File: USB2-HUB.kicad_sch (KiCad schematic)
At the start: 30 parts, among them IC2 TPS2553QDBVRQ1, IC7 TPS2553QDBVRQ1, J4 USB_C_Receptacle_USB2.0_16P, J5 USB_C_Receptacle_USB2.0_16P, U3 FSUSB42MUX

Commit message: layout draft
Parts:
- J4, J5: footprint (none) -> Connector_USB:USB_C_Receptacle_GCT_USB4105-xx-A_16P_TopMnt_Horizontal
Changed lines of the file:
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@@
 			)
 		)
-		(property "Footprint" ""
+		(property "Footprint" "Connector_USB:USB_C_Receptacle_GCT_USB4105-xx-A_16P_TopMnt_Horizontal"
 			(at 256.54 41.91 0)
 			(effects
@@
 			)
 		)
-		(property "Footprint" ""
+		(property "Footprint" "Connector_USB:USB_C_Receptacle_GCT_USB4105-xx-A_16P_TopMnt_Horizontal"
 			(at 256.54 116.84 0)
 			(effects

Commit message: moved everything to front & 0603'd stuff
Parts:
- C1, C12, C13, C15, C16, C17, C2, C4, C50, C57: footprint Capacitor_SMD:C_0805_2012Metric -> Capacitor_SMD:C_0603_1608Metric
- R10, R11, R12, R3, R37, R38, R5, R6, R62, R69, R9: footprint Resistor_SMD:R_0805_2012Metric -> Resistor_SMD:R_0603_1608Metric
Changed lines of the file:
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@@
 			)
 		)
-		(property "Footprint" "Capacitor_SMD:C_0805_2012Metric"
+		(property "Footprint" "Capacitor_SMD:C_0603_1608Metric"
 			(at 251.1552 149.86 0)
 			(effects
@@
 			)
 		)
-		(property "Footprint" "Resistor_SMD:R_0805_2012Metric"
+		(property "Footprint" "Resistor_SMD:R_0603_1608Metric"
 			(at 156.21 57.658 90)
 			(effects
@@
 			)
 		)
-		(property "Footprint" "Resistor_SMD:R_0805_2012Metric"
+		(property "Footprint" "Resistor_SMD:R_0603_1608Metric"
 			(at 204.978 57.15 90)
 			(effects
@@
 			)
 		)
-		(property "Footprint" "Resistor_SMD:R_0805_2012Metric"
+		(property "Footprint" "Resistor_SMD:R_0603_1608Metric"
 			(at 156.21 132.588 90)
 			(effects
@@
 			)
 		)
-		(property "Footprint" "Resistor_SMD:R_0805_2012Metric"
+		(property "Footprint" "Resistor_SMD:R_0603_1608Metric"
 			(at 241.3 29.972 90)
 			(effects
@@
 			)
 		)
-		(property "Footprint" "Capacitor_SMD:C_0805_2012Metric"
+		(property "Footprint" "Capacitor_SMD:C_0603_1608Metric"
 			(at 163.5252 64.77 0)
 			(effects
@@
 			)
 		)
-		(property "Footprint" "Capacitor_SMD:C_0805_2012Metric"
+		(property "Footprint" "Capacitor_SMD:C_0603_1608Metric"
 			(at 163.5252 139.7 0)
 			(effects
@@
 			)
 		)
-		(property "Footprint" "Resistor_SMD:R_0805_2012Metric"
+		(property "Footprint" "Resistor_SMD:R_0603_1608Metric"
 			(at 241.3 32.512 90)
 			(effects
@@
 			)
 		)
-		(property "Footprint" "Resistor_SMD:R_0805_2012Metric"
+		(property "Footprint" "Resistor_SMD:R_0603_1608Metric"
 			(at 241.3 104.902 90)
 			(effects
@@
 			)
 		)
-		(property "Footprint" "Resistor_SMD:R_0805_2012Metric"
+		(property "Footprint" "Resistor_SMD:R_0603_1608Metric"
 			(at 232.918 146.05 90)
 			(effects
@@
 			)
 		)
-		(property "Footprint" "Capacitor_SMD:C_0805_2012Metric"
+		(property "Footprint" "Capacitor_SMD:C_0603_1608Metric"
 			(at 240.9952 74.93 0)
 			(effects
@@
 			)
 		)
-		(property "Footprint" "Capacitor_SMD:C_0805_2012Metric"
+		(property "Footprint" "Capacitor_SMD:C_0603_1608Metric"
 			(at 166.0652 119.38 0)
 			(effects
@@
 			)
 		)
-		(property "Footprint" "Capacitor_SMD:C_0805_2012Metric"
+		(property "Footprint" "Capacitor_SMD:C_0603_1608Metric"
 			(at 214.3252 34.29 0)
 			(effects
@@
 			)
 		)
-		(property "Footprint" "Capacitor_SMD:C_0805_2012Metric"
+		(property "Footprint" "Capacitor_SMD:C_0603_1608Metric"
 			(at 251.1552 74.93 0)
 			(effects
@@
 			)
 		)
-		(property "Footprint" "Capacitor_SMD:C_0805_2012Metric"
+		(property "Footprint" "Capacitor_SMD:C_0603_1608Metric"
 			(at 166.0652 44.45 0)
 			(effects
@@
 			)
 		)
-		(property "Footprint" "Resistor_SMD:R_0805_2012Metric"
+		(property "Footprint" "Resistor_SMD:R_0603_1608Metric"
 			(at 241.3 107.442 90)
 			(effects
@@
 			)
 		)
-		(property "Footprint" "Capacitor_SMD:C_0805_2012Metric"
+		(property "Footprint" "Capacitor_SMD:C_0603_1608Metric"
 			(at 240.9952 149.86 0)
 			(effects
@@
 			)
 		)
-		(property "Footprint" "Resistor_SMD:R_0805_2012Metric"
+		(property "Footprint" "Resistor_SMD:R_0603_1608Metric"
 			(at 36.322 171.45 90)
 			(effects
@@
 			)
 		)
-		(property "Footprint" "Resistor_SMD:R_0805_2012Metric"
+		(property "Footprint" "Resistor_SMD:R_0603_1608Metric"
 			(at 204.978 132.08 90)
 			(effects
@@
 			)
 		)
-		(property "Footprint" "Resistor_SMD:R_0805_2012Metric"
+		(property "Footprint" "Resistor_SMD:R_0603_1608Metric"
 			(at 232.918 71.12 90)
 			(effects
@@
 			)
 		)
-		(property "Footprint" "Capacitor_SMD:C_0805_2012Metric"
+		(property "Footprint" "Capacitor_SMD:C_0603_1608Metric"
 			(at 214.3252 109.22 0)
 			(effects

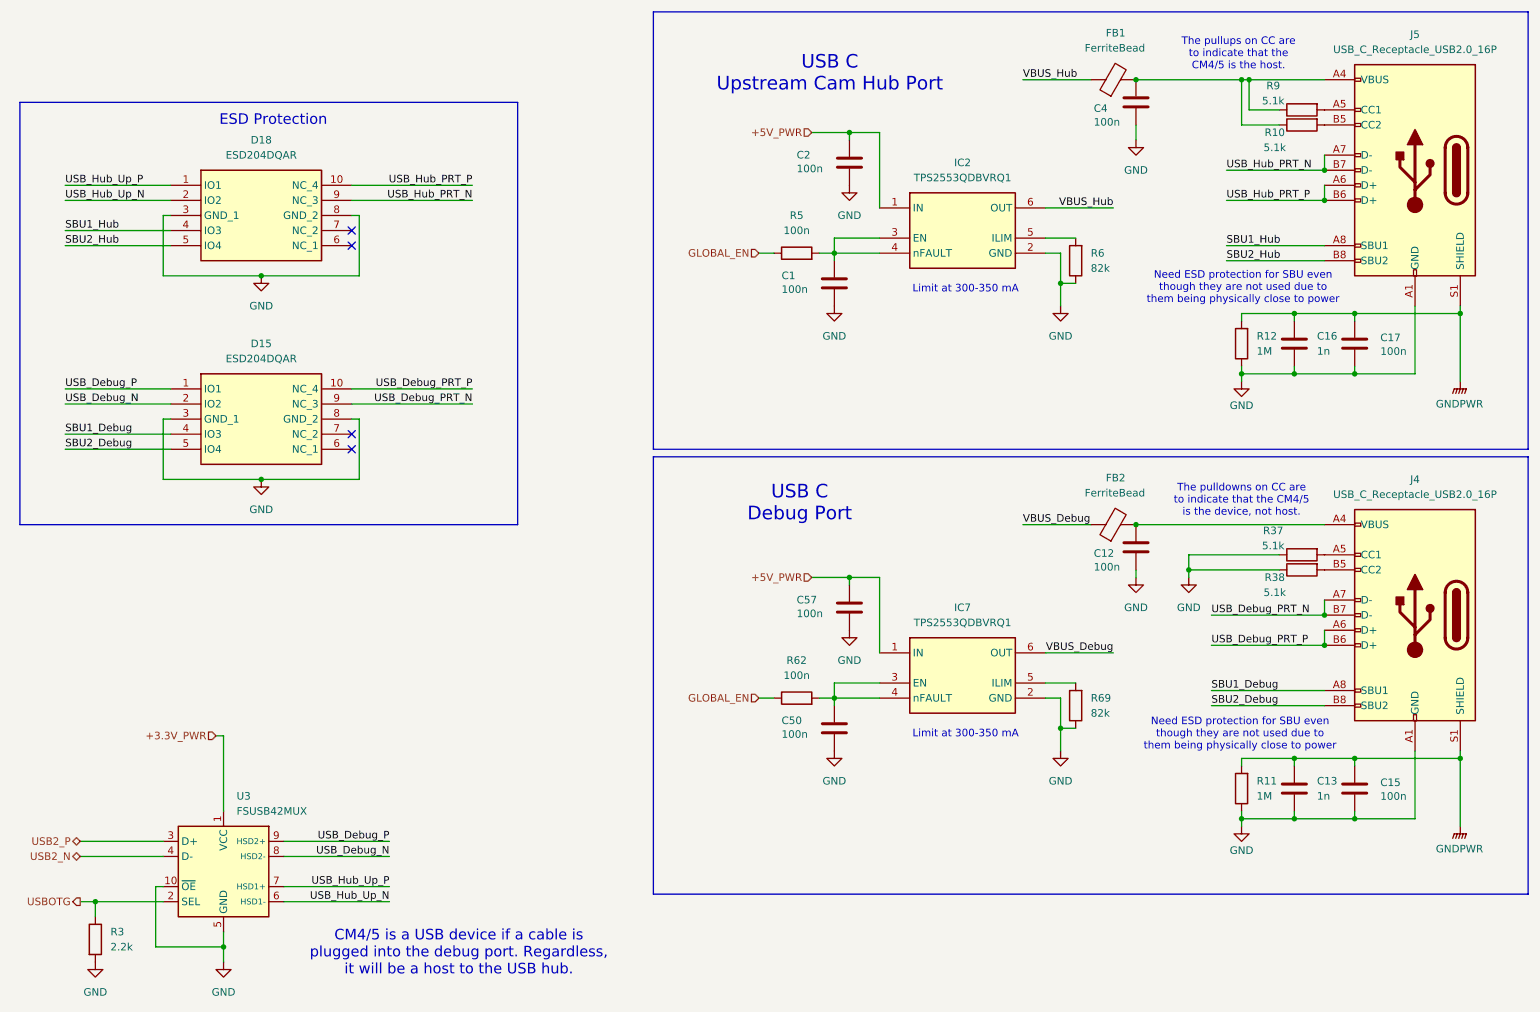
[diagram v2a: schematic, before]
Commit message: changed a bunch of stuff, still have work
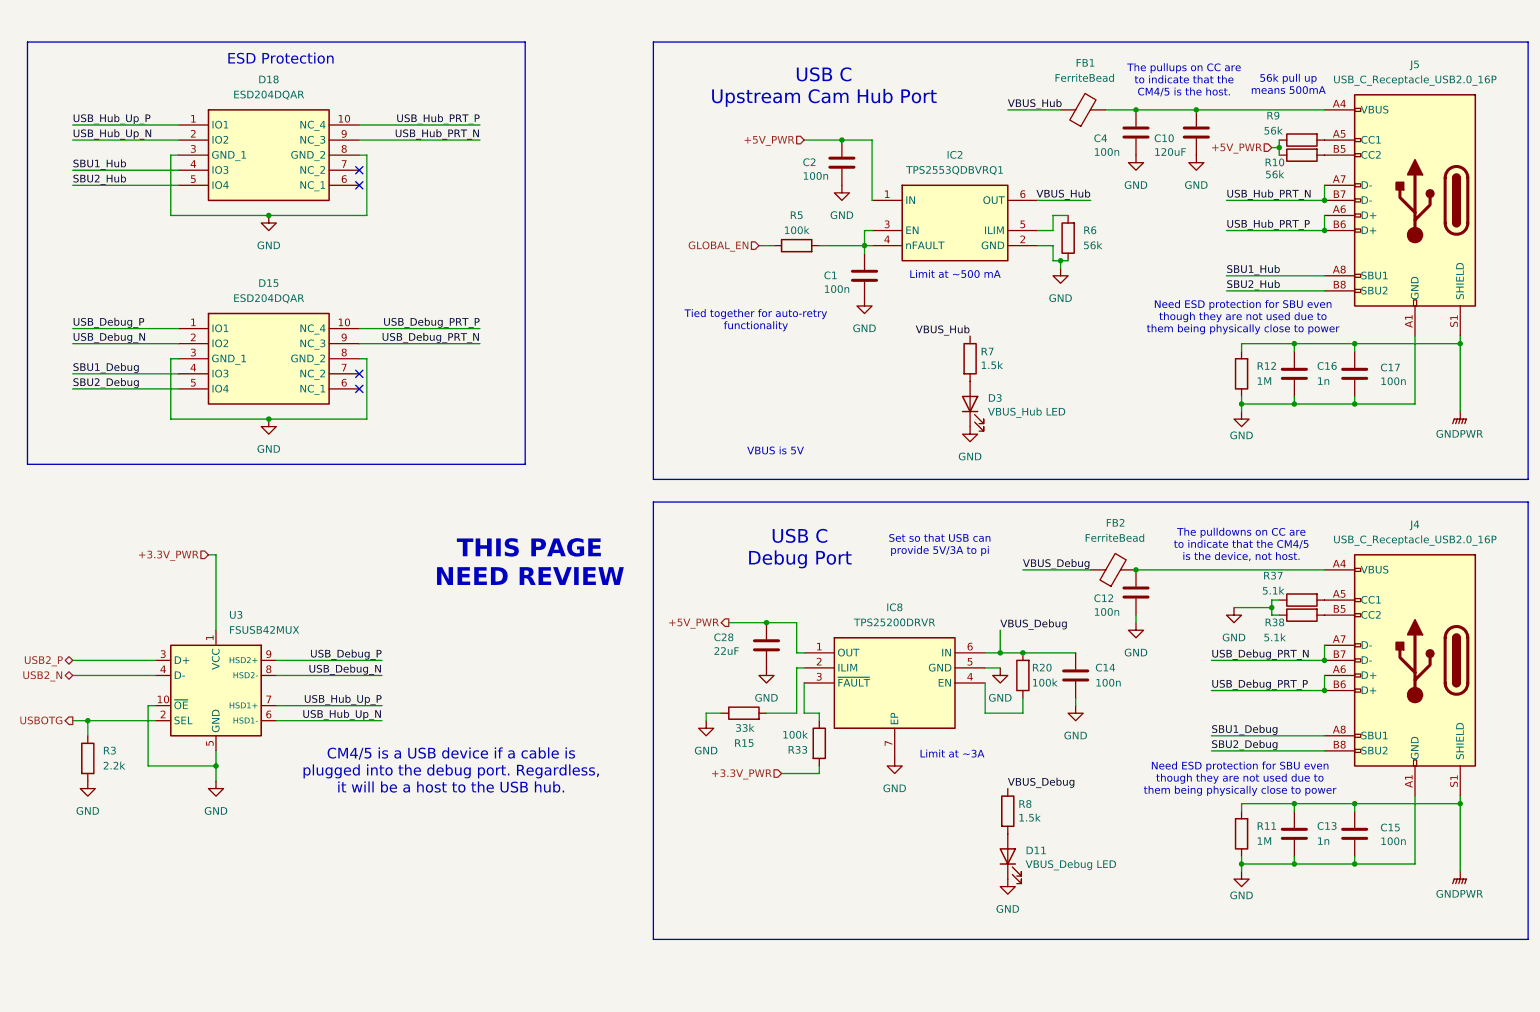
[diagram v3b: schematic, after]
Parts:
- removed C50, C57: 100n, Capacitor_SMD:C_0603_1608Metric, symbol Device:C
- removed IC7: TPS2553QDBVRQ1, Controls_Pi:SOT95P280X145-6N, symbol TPS2553QDBVRQ1:TPS2553QDBVRQ1
- removed R62: 100n, Resistor_SMD:R_0603_1608Metric, symbol Device:R
- removed R69: 82k, Resistor_SMD:R_0603_1608Metric, symbol Device:R
- added C10: 120uF, Capacitor_SMD:C_0603_1608Metric, symbol Device:C
- added C14: 100n, Capacitor_SMD:C_0603_1608Metric, symbol Device:C
- added C28: 22uF, Capacitor_SMD:C_0603_1608Metric, symbol Device:C
- added D11: VBUS_Debug LED, LED_SMD:LED_0603_1608Metric, symbol Device:LED
- added D3: VBUS_Hub LED, LED_SMD:LED_0603_1608Metric, symbol Device:LED
- added IC8: TPS25200DRVR, UTSVT_Power:SON65P200X200X80-7N, symbol TPS25200DRVR:TPS25200DRVR
- added R15: 33k, Resistor_SMD:R_0603_1608Metric, symbol Device:R
- added R20, R33: 100k, Resistor_SMD:R_0603_1608Metric, symbol Device:R
- added R7, R8: 1.5k, Resistor_SMD:R_0603_1608Metric, symbol Device:R
- R10, R9: value 5.1k -> 56k
- R5: value 100n -> 100k
- R6: value 82k -> 56k
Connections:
- net +3.3V_PWR: now also R33.2
- net +5V_PWR: now also R10.1, R9.1, C28.1, IC8.1 (OUT)
- net GND: now also C10.2, C14.2, C28.2, D11.1 (K), D3.1 (K), IC8.5 (GND), IC8.7 (EP), R15.1
- net VBUS_Debug: now also C14.1, IC8.6 (IN), R20.2, R8.1
- net VBUS_Hub: now also R7.1
- net at C4.1, FB1.2, J5.A4 (VBUS)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: now also C10.1; no longer R10.1, R9.1
- new net: D11.2 (A), R8.2
- new net: D3.2 (A), R7.2
- new net: IC8.3 (~{FAULT}), R33.1
- new net: IC8.2 (ILIM), R15.2
- new net: IC8.4 (EN), R20.1
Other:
- note added: "56k pull up means 500mA"
- note added: "Limit at ~3A"
- note added: "Limit at ~500 mA"
- note added: "Set so that USB can provide 5V/3A to pi"
- note added: "THIS PAGE NEED REVIEW"
- note added: "Tied together for auto-retry functionality"
- note added: "VBUS is 5V"
- note removed: "Limit at 300-350 mA"
- moved on the sheet: C1, C12, C13, C15, C16, C17, C2, D15, D18, FB1, FB2, IC2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
